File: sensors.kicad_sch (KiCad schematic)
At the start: 14 parts, among them U5 BMI088, U6 MS5611-01BA, U7 LIS2MDL, U8 SHT4x

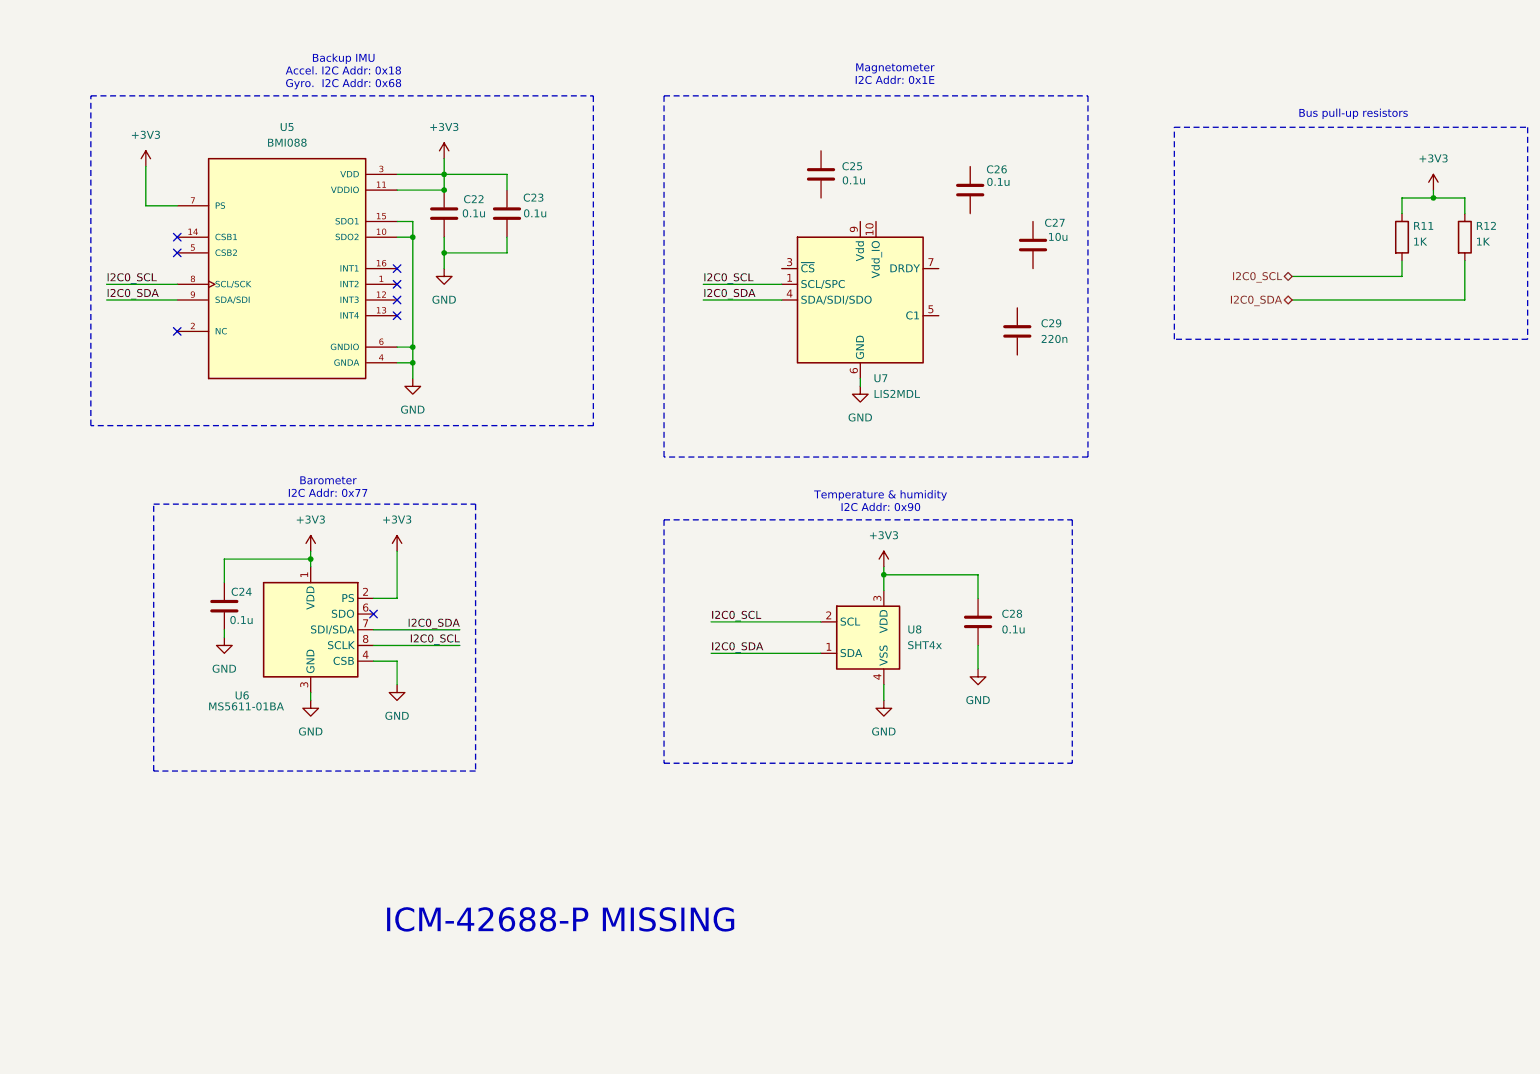
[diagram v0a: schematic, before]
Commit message: nearly completed schematic, partial layout
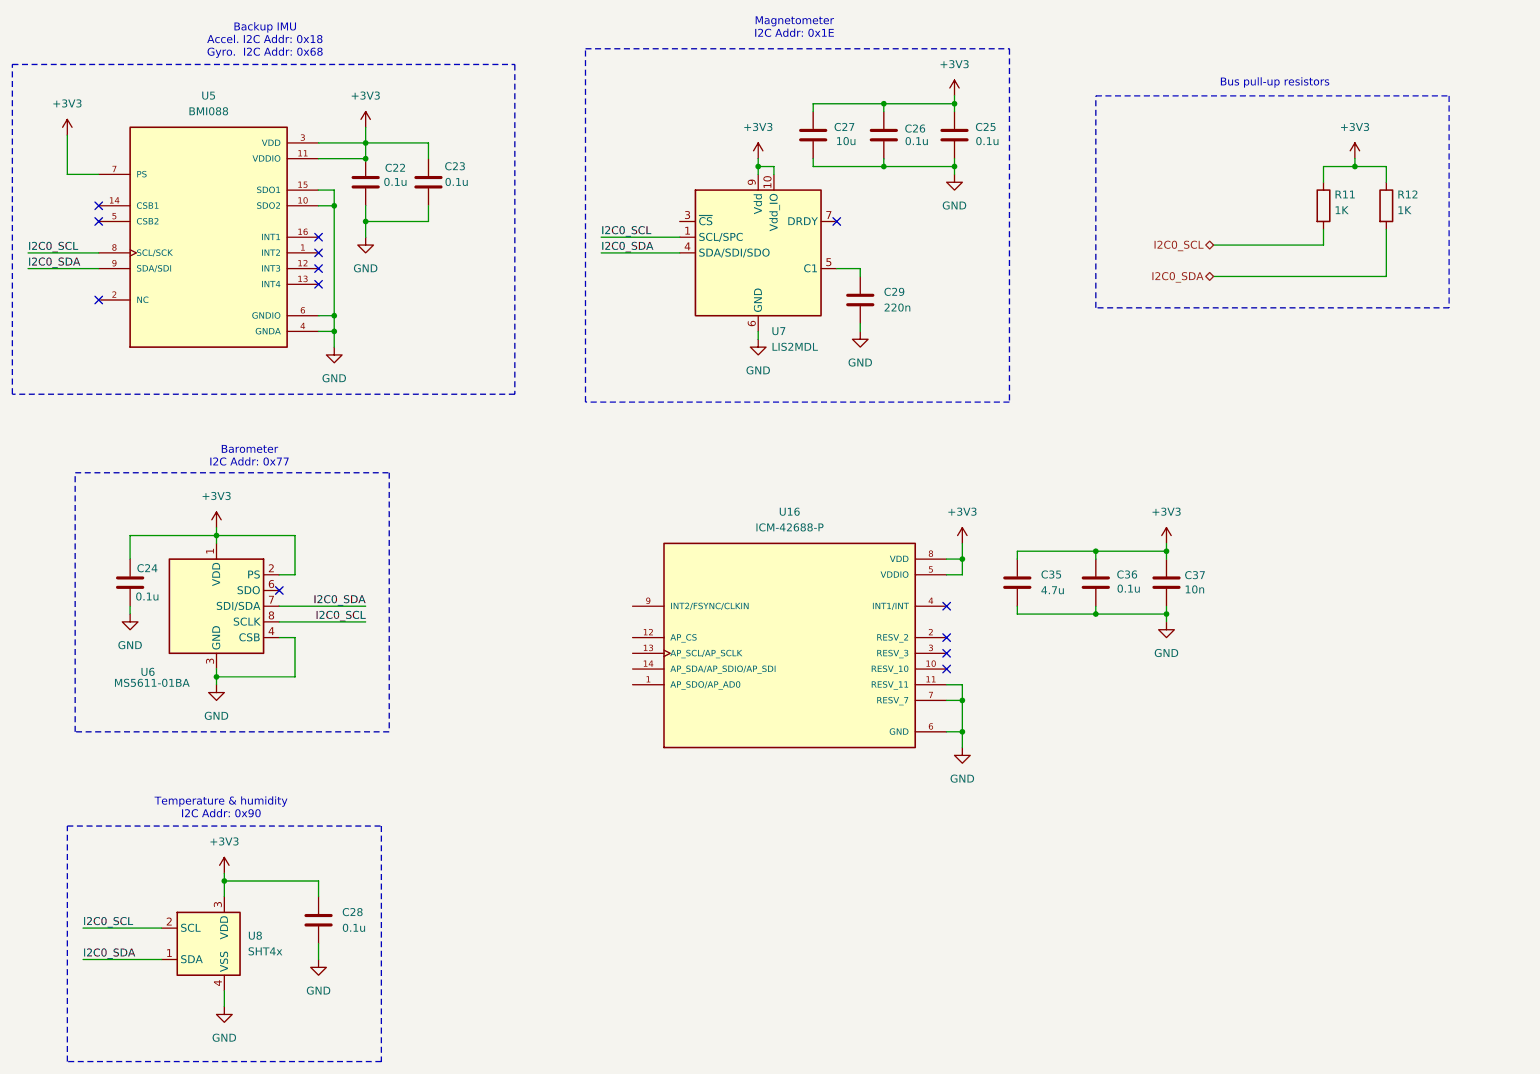
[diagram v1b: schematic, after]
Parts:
- added C35: 4.7u, Capacitor_SMD:C_0805_2012Metric, symbol Device:C
- added C36: 0.1u, Capacitor_SMD:C_0603_1608Metric, symbol Device:C
- added C37: 10n, Capacitor_SMD:C_0603_1608Metric, symbol Device:C
- added U16: ICM-42688-P, LRI_partlib:IIM42352, symbol LRI_partlib:ICM-42688-P
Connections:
- net +3V3: now also C25.2, C26.1, C27.2, U7.10 (Vdd_IO), U7.9 (Vdd), C35.1, C36.2, C37.1, U16.5 (VDDIO), U16.8 (VDD)
- net GND: now also C25.1, C26.2, C27.1, C29.2, C35.2, C36.1, C37.2, U16.11 (RESV_11), U16.6 (GND), U16.7 (RESV_7)
- net at C29.1: now also U7.5 (C1)
- no-connect marks 8 -> 13
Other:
- note removed: "ICM-42688-P MISSING"
- moved on the sheet: C22, C23, C24, C25, C26, C28, C29, R11, R12, U5, U6, U7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
